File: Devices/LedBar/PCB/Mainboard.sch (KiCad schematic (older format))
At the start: 4 parts

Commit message: Many small fixes
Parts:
- H203: footprint MountingHole:MountingHole_4.3mm_M4 -> AmbientLight:MountingHole_4.3mm_M4_modified1
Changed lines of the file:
@@
 F 0 "H203" H 9600 1546 50  0000 L CNN
 F 1 "MountingHole" H 9600 1455 50  0000 L CNN
-F 2 "MountingHole:MountingHole_4.3mm_M4" H 9500 1500 50  0001 C CNN
+F 2 "AmbientLight:MountingHole_4.3mm_M4_modified1" H 9500 1500 50  0001 C CNN
 F 3 "~" H 9500 1500 50  0001 C CNN
 	1    9500 1500

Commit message: Renamed libraries
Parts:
- H203: footprint AmbientLight:MountingHole_4.3mm_M4_modified1 -> RGBW-Bar:MountingHole_4.3mm_M4_modified1
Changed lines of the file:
@@
 F 0 "H203" H 9600 1546 50  0000 L CNN
 F 1 "MountingHole" H 9600 1455 50  0000 L CNN
-F 2 "AmbientLight:MountingHole_4.3mm_M4_modified1" H 9500 1500 50  0001 C CNN
+F 2 "RGBW-Bar:MountingHole_4.3mm_M4_modified1" H 9500 1500 50  0001 C CNN
 F 3 "~" H 9500 1500 50  0001 C CNN
 	1    9500 1500

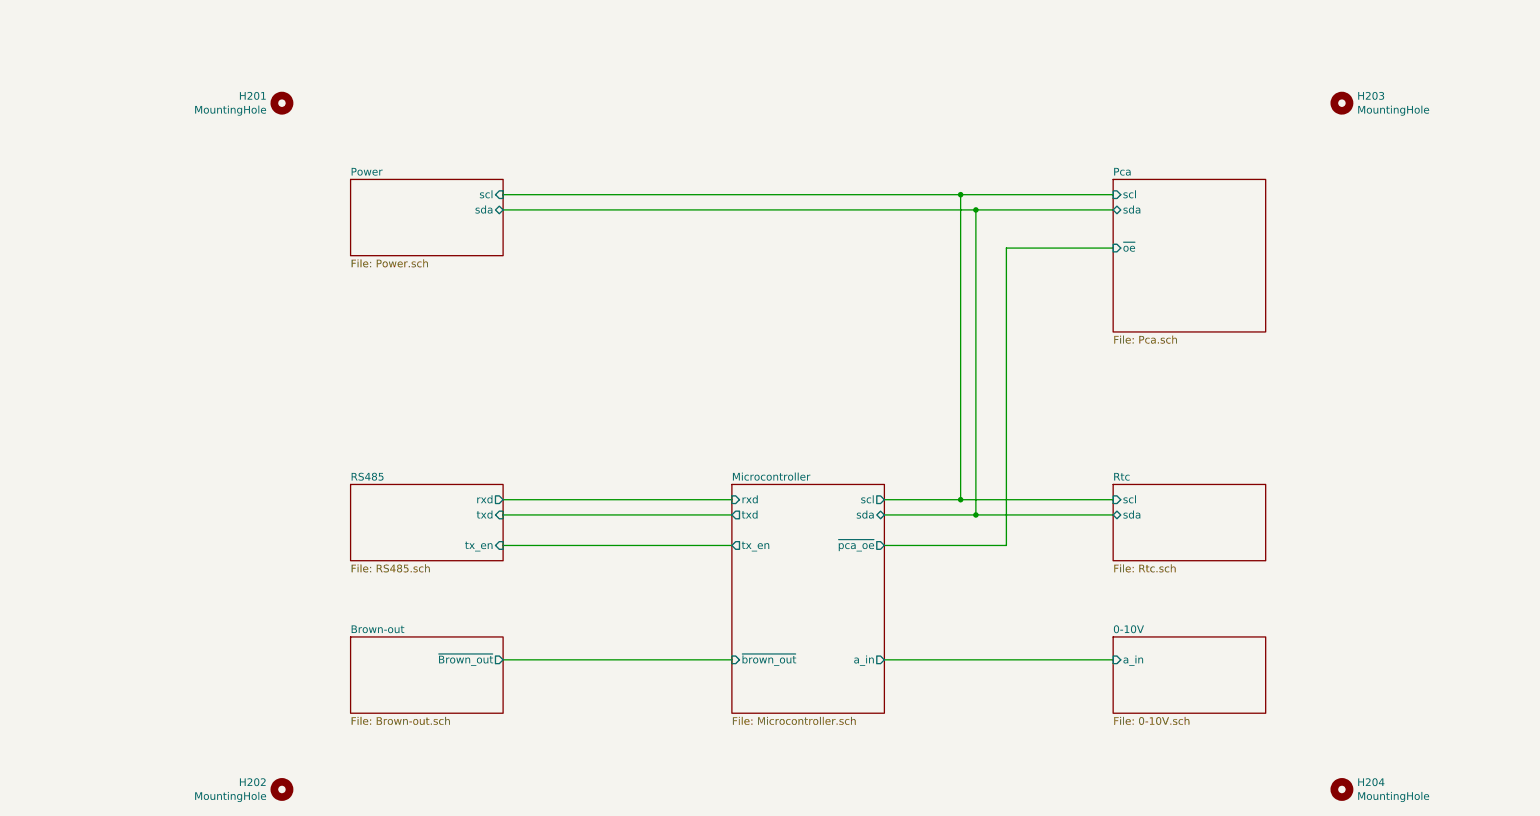
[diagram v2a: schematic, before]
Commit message: Cosmetic changes to shematics
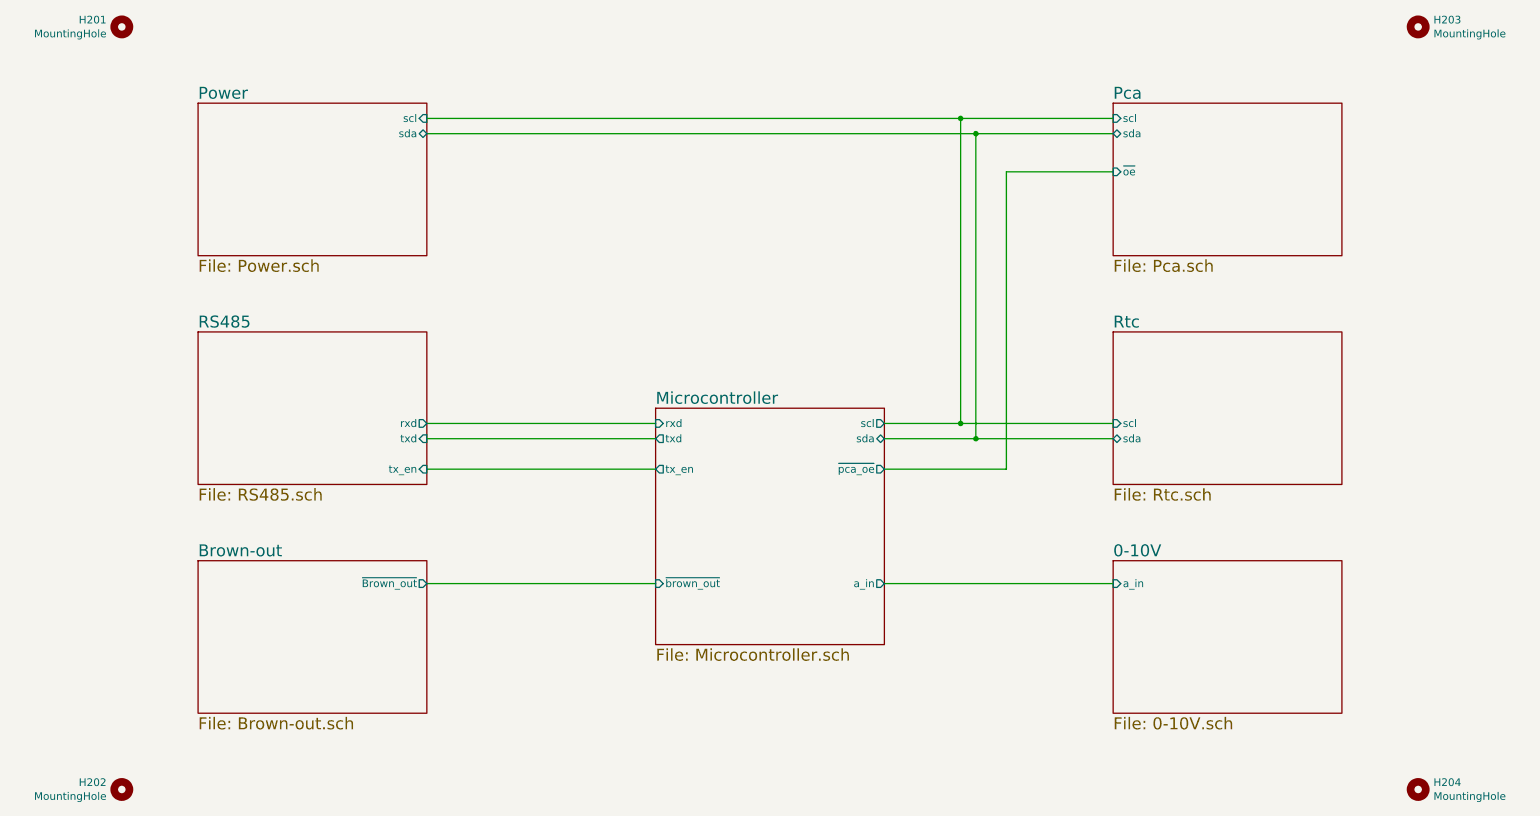
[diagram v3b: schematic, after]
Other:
- moved on the sheet: H201, H202, H203, H204
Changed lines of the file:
@@
 Rev "0.1"
 Comp "Roel Drost"
-Comment1 ""
+Comment1 "GNU General Public License v3.0"
 Comment2 ""
 Comment3 ""
-Comment4 ""
+Comment4 "4 channel RGBW LED bar, Arduino compatible with isolated half duplex RS485."
 $EndDescr
 $Sheet
-S 3000 2000 1000 500
+S 2000 1500 1500 1000
 U 60858D7F
-F0 "Power" 50
-F1 "Power.sch" 50
-F2 "scl" I R 4000 2100 50
-F3 "sda" B R 4000 2200 50
-$EndSheet
-$Sheet
-S 3000 4000 1000 500
-U 608655BB
-F0 "RS485" 50
-F1 "RS485.sch" 50
-F2 "txd" I R 4000 4200 50
-F3 "rxd" O R 4000 4100 50
-F4 "tx_en" I R 4000 4400 50
+F0 "Power" 78
+F1 "Power.sch" 78
+F2 "scl" I R 3500 1600 50
+F3 "sda" B R 3500 1700 50
 $EndSheet
 Wire Wire Line
-	7000 2100 7000 4100
+	7000 1600 7000 3600
 Wire Wire Line
-	7000 4100 6500 4100
+	7000 3600 6500 3600
 Wire Wire Line
-	7100 2200 7100 4200
+	7100 1700 7100 3700
 Wire Wire Line
-	7100 4200 6500 4200
+	7100 3700 6500 3700
 Wire Wire Line
-	6500 4400 7300 4400
+	6500 3900 7300 3900
+Connection ~ 7000 1600
+Wire Wire Line
+	7000 1600 8000 1600
+Wire Wire Line
+	7100 1700 8000 1700
+Connection ~ 7100 1700
+Wire Wire Line
+	8000 1950 7300 1950
+Wire Wire Line
+	7300 1950 7300 3900
 $Sheet
-S 8000 2000 1000 1000
-U 608B2A01
-F0 "Pca" 50
-F1 "Pca.sch" 50
-F2 "scl" I L 8000 2100 50
-F3 "sda" B L 8000 2200 50
-F4 "~oe~" I L 8000 2450 50
-$EndSheet
-Connection ~ 7000 2100
-Wire Wire Line
-	7000 2100 8000 2100
-Wire Wire Line
-	7100 2200 8000 2200
-Connection ~ 7100 2200
-Wire Wire Line
-	8000 2450 7300 2450
-Wire Wire Line
-	7300 2450 7300 4400
-$Sheet
-S 8000 5000 1000 500
+S 8000 4500 1500 1000
 U 608C0E66
-F0 "0-10V" 50
-F1 "0-10V.sch" 50
-F2 "a_in" I L 8000 5150 50
+F0 "0-10V" 78
+F1 "0-10V.sch" 78
+F2 "a_in" I L 8000 4650 50
 $EndSheet
 Wire Wire Line
-	6500 5150 8000 5150
+	6500 4650 8000 4650
 $Sheet
-S 5500 4000 1000 1500
-U 608B1159
-F0 "Microcontroller" 50
-F1 "Microcontroller.sch" 50
-F2 "rxd" I L 5500 4100 50
-F3 "txd" O L 5500 4200 50
-F4 "tx_en" O L 5500 4400 50
-F5 "~pca_oe~" O R 6500 4400 50
-F6 "scl" O R 6500 4100 50
-F7 "sda" B R 6500 4200 50
-F8 "~brown_out~" I L 5500 5150 50
-F9 "a_in" O R 6500 5150 50
-$EndSheet
-$Sheet
-S 3000 5000 1000 500
+S 2000 4500 1500 1000
 U 6094F41A
-F0 "Brown-out" 50
-F1 "Brown-out.sch" 50
-F2 "~Brown_out~" O R 4000 5150 50
+F0 "Brown-out" 78
+F1 "Brown-out.sch" 78
+F2 "~Brown_out~" O R 3500 4650 50
 $EndSheet
 Wire Wire Line
-	4000 2100 7000 2100
+	3500 3600 5000 3600
 Wire Wire Line
-	4000 2200 7100 2200
+	3500 3700 5000 3700
 Wire Wire Line
-	4000 4100 5500 4100
+	3500 3900 5000 3900
 Wire Wire Line
-	4000 4200 5500 4200
-Wire Wire Line
-	4000 4400 5500 4400
-Wire Wire Line
-	4000 5150 5500 5150
-$Comp
-L Mechanical:MountingHole H201
-U 1 1 6174F005
-P 2550 1500
-F 0 "H201" H 2650 1546 50  0000 L CNN
-F 1 "MountingHole" H 2650 1455 50  0000 L CNN
-F 2 "MountingHole:MountingHole_4.3mm_M4" H 2550 1500 50  0001 C CNN
-F 3 "~" H 2550 1500 50  0001 C CNN
-	1    2550 1500
-	-1   0    0    -1
-$EndComp
-$Comp
-L Mechanical:MountingHole H203
-U 1 1 617508E9
-P 9500 1500
-F 0 "H203" H 9600 1546 50  0000 L CNN
-F 1 "MountingHole" H 9600 1455 50  0000 L CNN
-F 2 "RGBW-Bar:MountingHole_4.3mm_M4_modified1" H 9500 1500 50  0001 C CNN
-F 3 "~" H 9500 1500 50  0001 C CNN
-	1    9500 1500
-	1    0    0    -1
-$EndComp
+	3500 4650 5000 4650
 $Comp
 L Mechanical:MountingHole H204
 U 1 1 61B9622B
-P 9500 6000
-F 0 "H204" H 9600 6046 50  0000 L CNN
-F 1 "MountingHole" H 9600 5955 50  0000 L CNN
-F 2 "MountingHole:MountingHole_4.3mm_M4" H 9500 6000 50  0001 C CNN
-F 3 "~" H 9500 6000 50  0001 C CNN
-	1    9500 6000
+P 10000 6000
+F 0 "H204" H 10100 6046 50  0000 L CNN
+F 1 "MountingHole" H 10100 5955 50  0000 L CNN
+F 2 "MountingHole:MountingHole_4.3mm_M4" H 10000 6000 50  0001 C CNN
+F 3 "~" H 10000 6000 50  0001 C CNN
+	1    10000 6000
 	1    0    0    -1
 $EndComp
@@
 L Mechanical:MountingHole H202
 U 1 1 61B96485
-P 2550 6000
-F 0 "H202" H 2650 6046 50  0000 L CNN
-F 1 "MountingHole" H 2650 5955 50  0000 L CNN
-F 2 "MountingHole:MountingHole_4.3mm_M4" H 2550 6000 50  0001 C CNN
-F 3 "~" H 2550 6000 50  0001 C CNN
-	1    2550 6000
+P 1500 6000
+F 0 "H202" H 1600 6046 50  0000 L CNN
+F 1 "MountingHole" H 1600 5955 50  0000 L CNN
+F 2 "MountingHole:MountingHole_4.3mm_M4" H 1500 6000 50  0001 C CNN
+F 3 "~" H 1500 6000 50  0001 C CNN
+	1    1500 6000
 	-1   0    0    -1
 $EndComp
 $Sheet
-S 8000 4000 1000 500
+S 8000 3000 1500 1000
 U 61792A36
-F0 "Rtc" 50
-F1 "Rtc.sch" 50
-F2 "scl" I L 8000 4100 50
-F3 "sda" B L 8000 4200 50
+F0 "Rtc" 78
+F1 "Rtc.sch" 78
+F2 "scl" I L 8000 3600 50
+F3 "sda" B L 8000 3700 50
 $EndSheet
 Wire Wire Line
-	7000 4100 8000 4100
-Connection ~ 7000 4100
+	7000 3600 8000 3600
+Connection ~ 7000 3600
 Wire Wire Line
-	8000 4200 7100 4200
-Connection ~ 7100 4200
+	8000 3700 7100 3700
+Connection ~ 7100 3700
+$Sheet
+S 5000 3500 1500 1550
+U 608B1159
+F0 "Microcontroller" 78
+F1 "Microcontroller.sch" 78
+F2 "rxd" I L 5000 3600 50
+F3 "txd" O L 5000 3700 50
+F4 "tx_en" O L 5000 3900 50
+F5 "~pca_oe~" O R 6500 3900 50
+F6 "scl" O R 6500 3600 50
+F7 "sda" B R 6500 3700 50
+F8 "~brown_out~" I L 5000 4650 50
+F9 "a_in" O R 6500 4650 50
+$EndSheet
+$Sheet
+S 8000 1500 1500 1000
+U 608B2A01
+F0 "Pca" 78
+F1 "Pca.sch" 78
+F2 "scl" I L 8000 1600 50
+F3 "sda" B L 8000 1700 50
+F4 "~oe~" I L 8000 1950 50
+$EndSheet
+$Sheet
+S 2000 3000 1500 1000
+U 608655BB
+F0 "RS485" 78
+F1 "RS485.sch" 78
+F2 "txd" I R 3500 3700 50
+F3 "rxd" O R 3500 3600 50
+F4 "tx_en" I R 3500 3900 50
+$EndSheet
+Wire Wire Line
+	3500 1600 7000 1600
+Wire Wire Line
+	3500 1700 7100 1700
+$Comp
+L Mechanical:MountingHole H203
+U 1 1 617508E9
+P 10000 1000
+F 0 "H203" H 10100 1046 50  0000 L CNN
+F 1 "MountingHole" H 10100 955 50  0000 L CNN
+F 2 "RGBW-Bar:MountingHole_4.3mm_M4_modified1" H 10000 1000 50  0001 C CNN
+F 3 "~" H 10000 1000 50  0001 C CNN
+	1    10000 1000
+	1    0    0    -1
+$EndComp
+$Comp
+L Mechanical:MountingHole H201
+U 1 1 6174F005
+P 1500 1000
+F 0 "H201" H 1600 1046 50  0000 L CNN
+F 1 "MountingHole" H 1600 955 50  0000 L CNN
+F 2 "MountingHole:MountingHole_4.3mm_M4" H 1500 1000 50  0001 C CNN
+F 3 "~" H 1500 1000 50  0001 C CNN
+	1    1500 1000
+	-1   0    0    -1
+$EndComp
 $EndSCHEMATC
